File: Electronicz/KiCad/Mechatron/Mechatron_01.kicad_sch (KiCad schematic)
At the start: 54 parts, among them J1 Conn_01x15_Socket, J10 Servo_1, J11 Servo_2, J12 Servo_3, J13 V_ESP32, J14 GND_ESP32, J15 Motor_1, J16 Motor_2, J17 Motor_3, J18 Motor_4, J19 V_LED_2, J2 Front, J20 V_LED_1, J21 V_LED_top, J22 GND_LED_top, J23 GND_LED_2, J24 GND_LED_1, J25 SD-Card-Reader, J26 AUDIOAMP, J27 Speaker, J28 Conn_01x01_Pin, J29 Conn_01x01_Pin, J3 Left_Front, J30 SW, J4 Left_Back, J5 Back, J6 Right_Back, J7 Right_Front, J8 GND_Battery, J9 V_Battery_Switch, Q1 LR_LED_Sensors, Q2 LR_3, Q3 LR_2, Q4 LR_1, Q5 LED_top, Q6 LED_2, Q7 LED_1

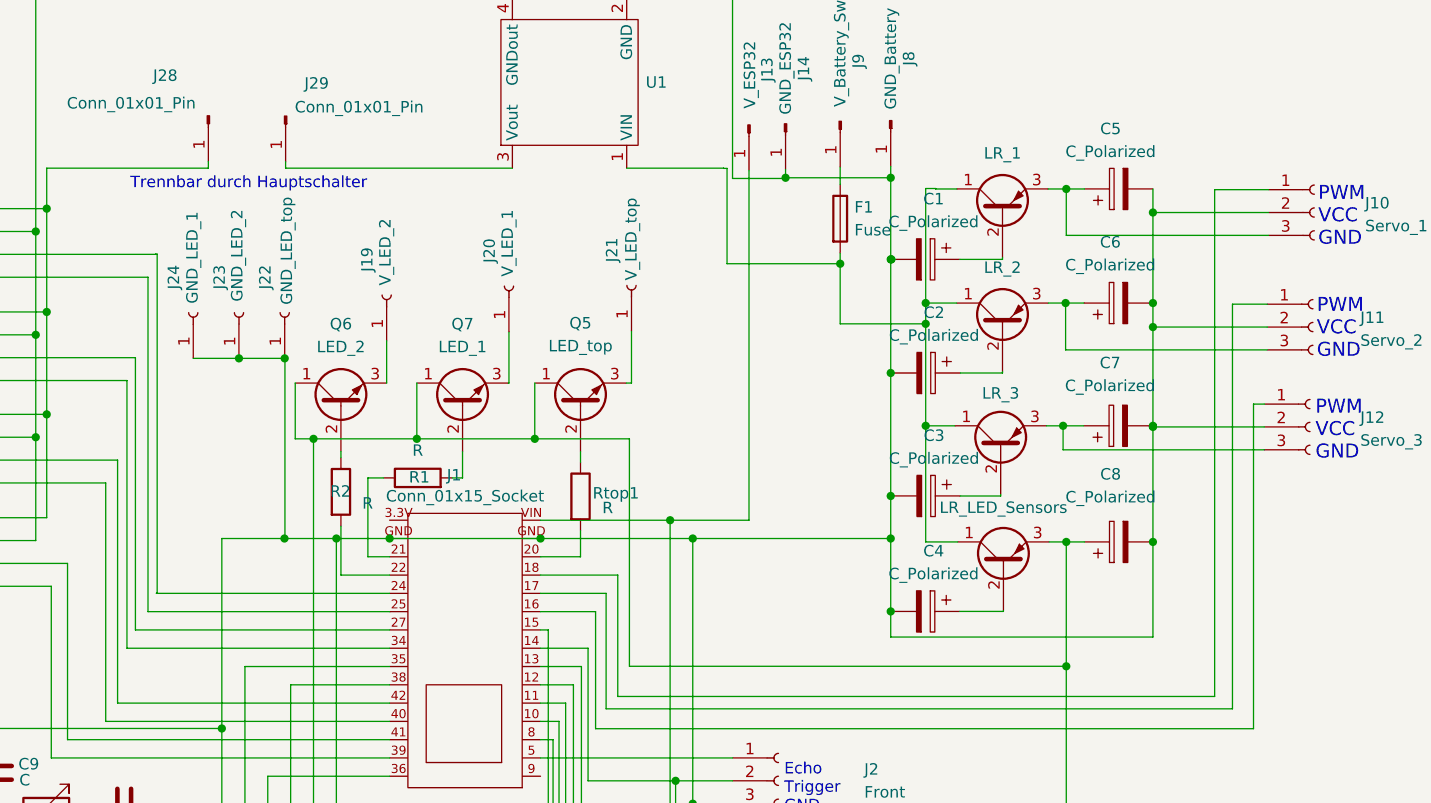
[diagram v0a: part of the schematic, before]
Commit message: Finishing PCB
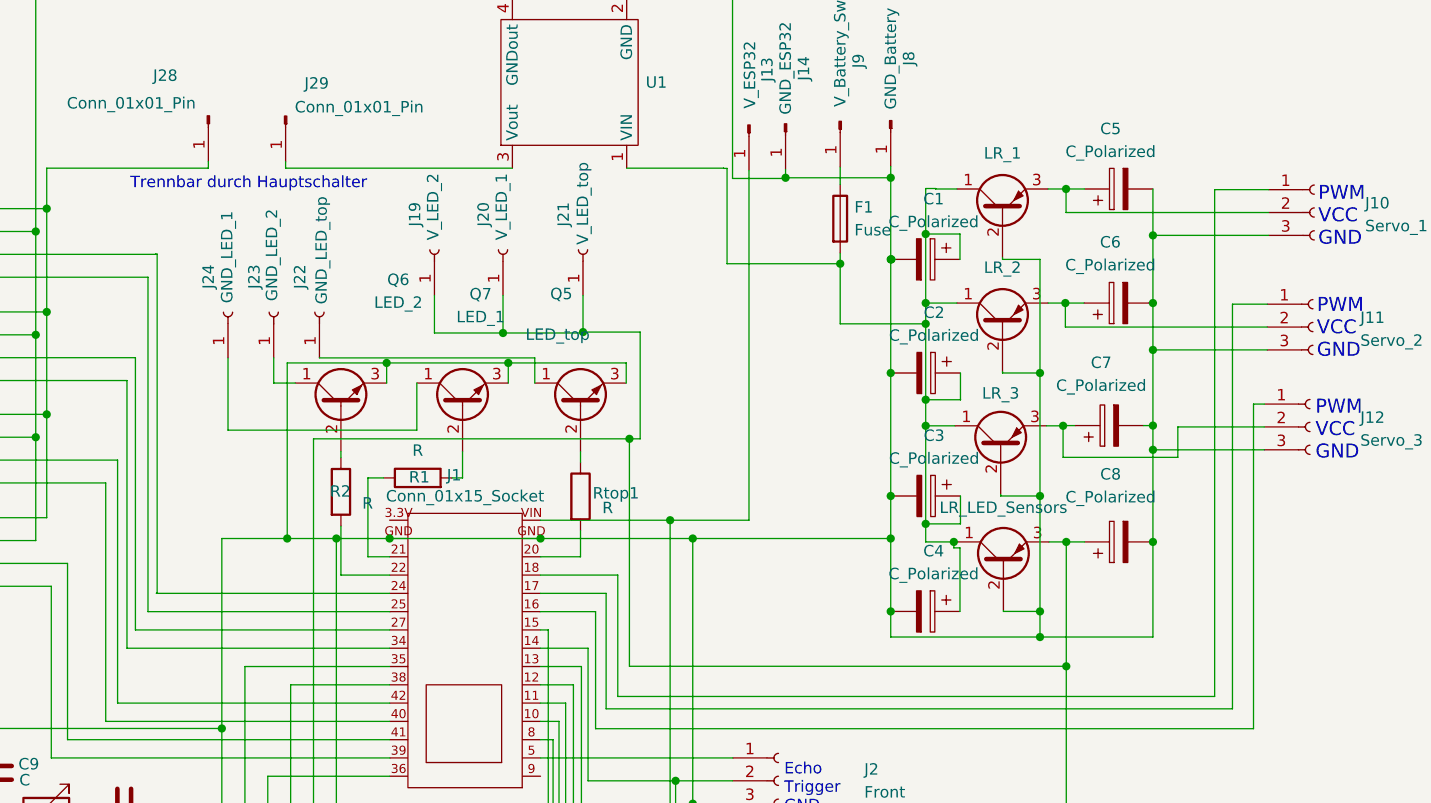
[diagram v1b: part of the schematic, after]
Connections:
- net at C1.2, C2.2, C3.2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: now also J10.3 (Pin_3), J11.3 (Pin_3), J12.3 (Pin_3), Q1.2 (B), Q2.2 (B), Q3.2 (B), Q4.2 (B), Q5.3 (E), Q6.3 (E), Q7.3 (E); no longer J10.2 (Pin_2), J11.2 (Pin_2), J12.2 (Pin_2), J22.1 (Pin_1), J23.1 (Pin_1), J24.1 (Pin_1)
- net at C8.1, J2.4 (Pin_4), J25.2 (Pin_2)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: now also J19.1 (Pin_1), J20.1 (Pin_1), J21.1 (Pin_1); no longer Q5.1 (C), Q6.1 (C), Q7.1 (C)
- net at C6.1, Q3.3 (E): now also J11.2 (Pin_2); no longer J11.3 (Pin_3)
- net at C1.1: now also C2.1, C3.1, C4.1, F1.2, Q1.1 (C), Q2.1 (C), Q3.1 (C), Q4.1 (C), U1.1 (VIN); no longer Q4.2 (B)
- net at C5.1, Q4.3 (E): now also J10.2 (Pin_2); no longer J10.3 (Pin_3)
- net at C7.1, Q2.3 (E): now also J12.2 (Pin_2); no longer J12.3 (Pin_3)
- new net: J24.1 (Pin_1), Q7.1 (C)
- new net: J22.1 (Pin_1), Q5.1 (C)
- new net: J23.1 (Pin_1), Q6.1 (C)
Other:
- moved on the sheet: C7, J19, J20, J21, J22, J23, J24
